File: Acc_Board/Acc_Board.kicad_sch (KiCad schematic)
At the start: 52 parts, among them J1 AIRs Power, J12 776087-1, J3 IMD BAT, J4 HV Power, J5 HVIL, J6 IMD, J7 Current Sensor, J8 Fans, J9 Shutdown IL, K1 Relay_SPST-NO, Q1 STS6NF20V, Q2 STS6NF20V, Q3 STS6NF20V, U1 ISO1050DUB, U15 MCP6004, U2 NUCLEO-L432KC, U4 PQDE6W-Q110-S5-H-D, U5 R-78B5.0-2.0, U8 LM7809_TO220

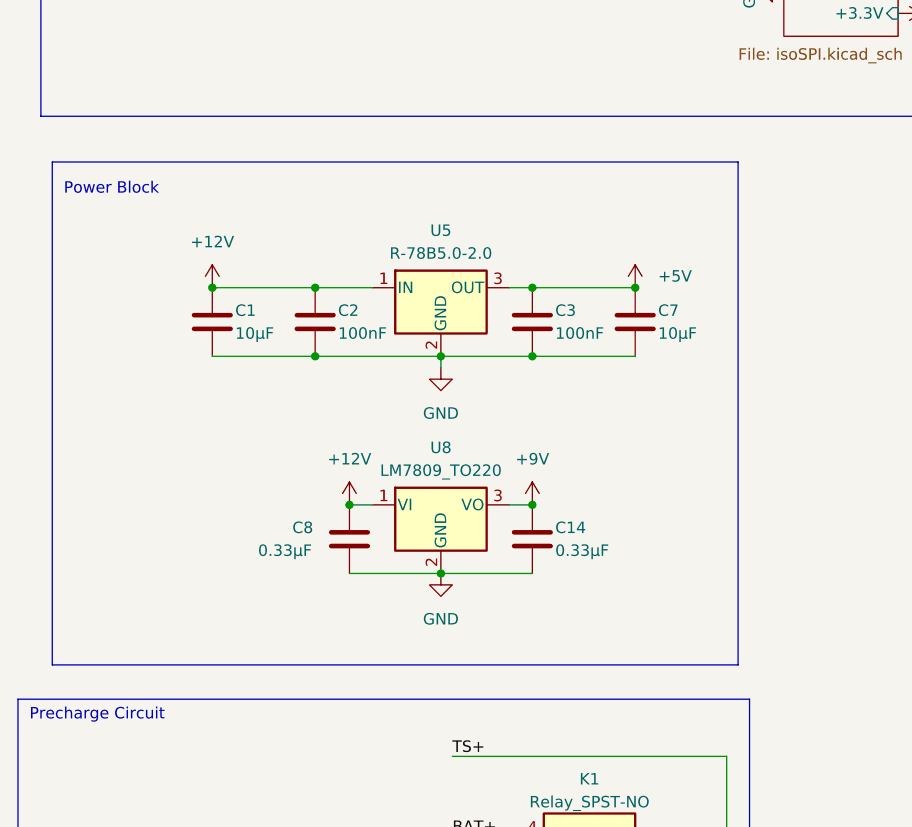
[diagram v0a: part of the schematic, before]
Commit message: Acc board traces done (for now)
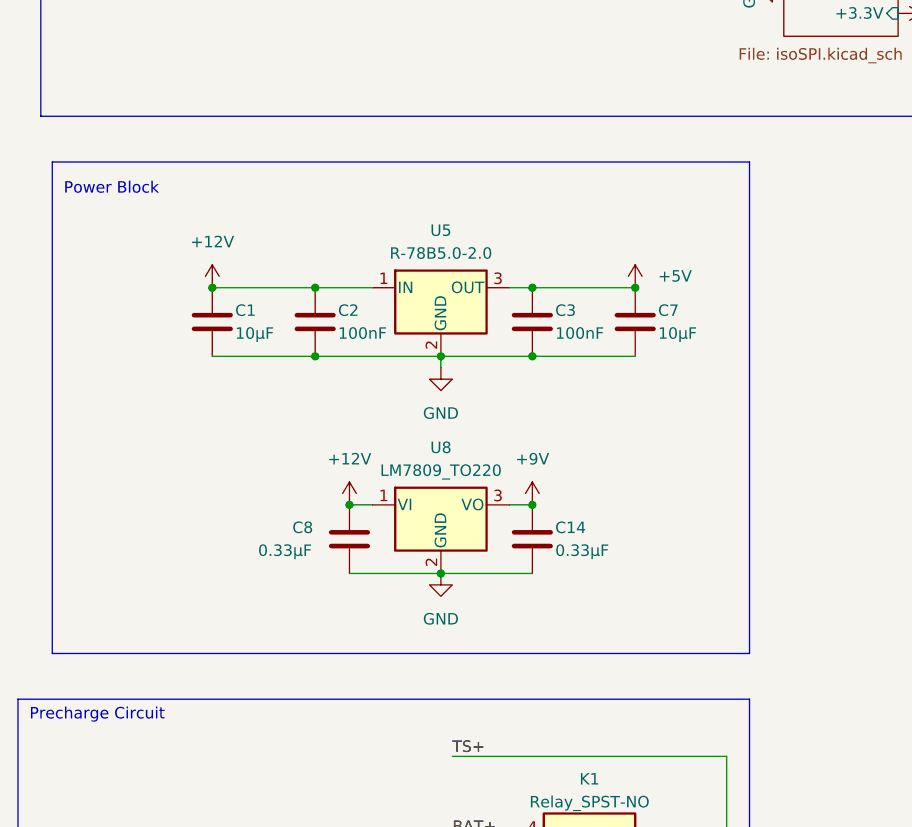
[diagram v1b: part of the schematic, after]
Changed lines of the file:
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@@
     (fill (type none))
   )
-  (rectangle (start 24.13 115.57) (end 100.33 171.45)
+  (rectangle (start 24.13 115.57) (end 101.6 170.18)
     (stroke (width 0) (type default))
     (fill (type none))
